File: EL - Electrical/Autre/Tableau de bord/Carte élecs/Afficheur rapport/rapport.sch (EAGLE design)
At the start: 15 parts, among them IC1 MCP23008P, X1 22-23-2041

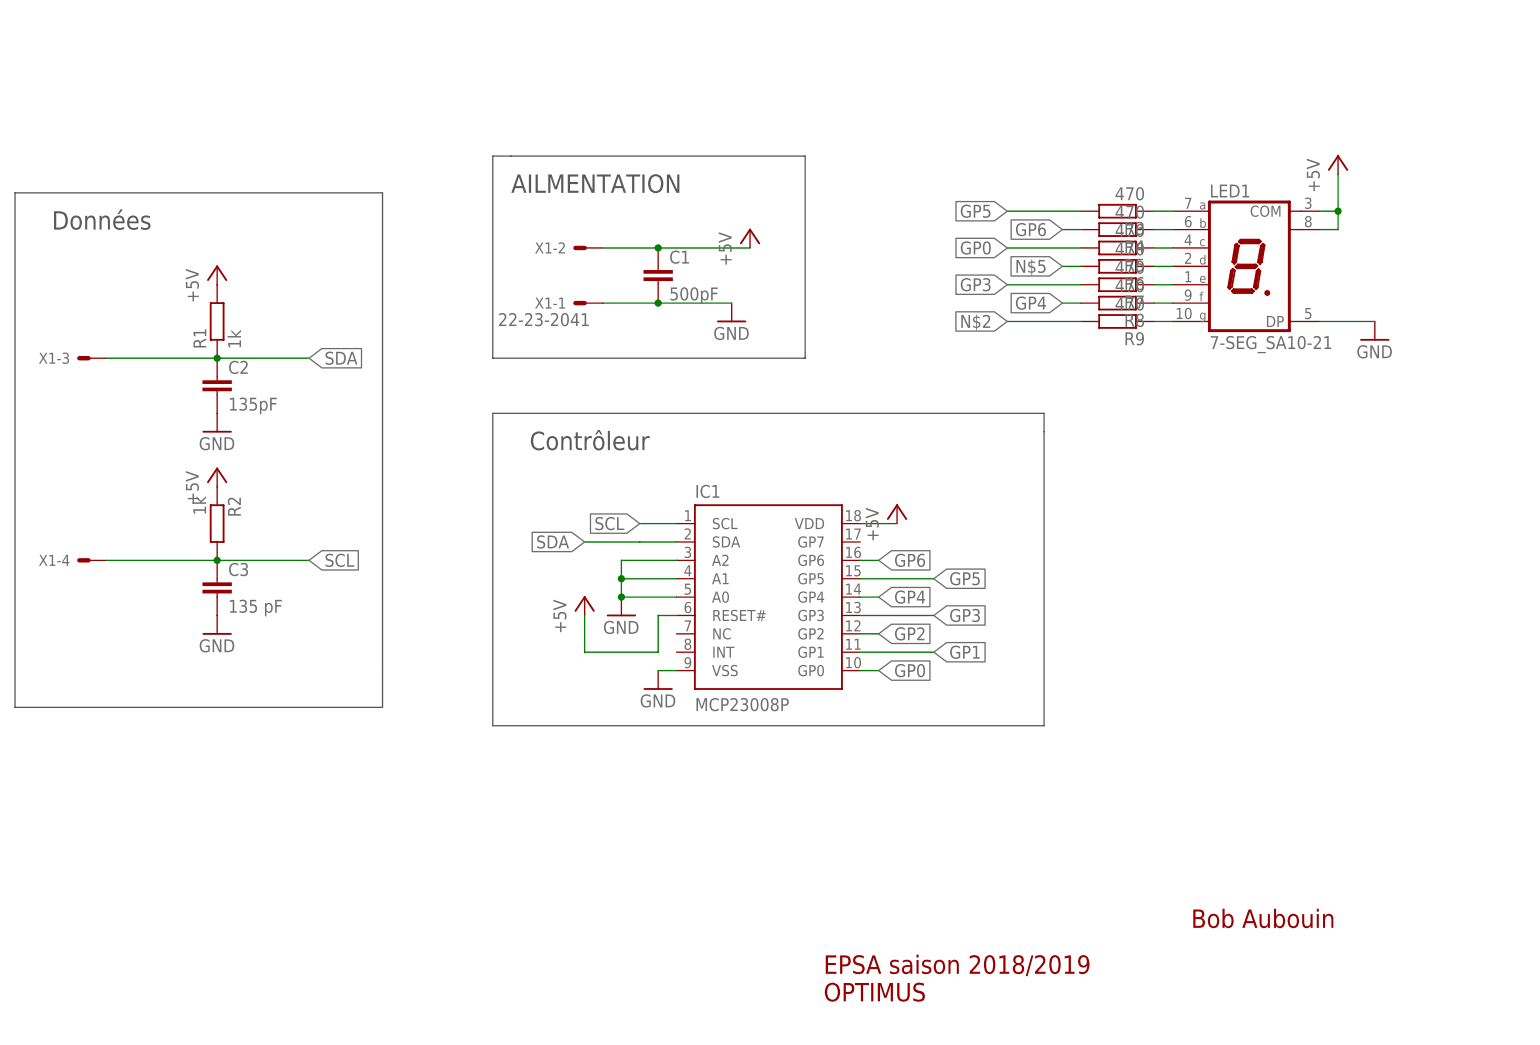
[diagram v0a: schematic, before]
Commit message: carte afficheur rapport et commandes
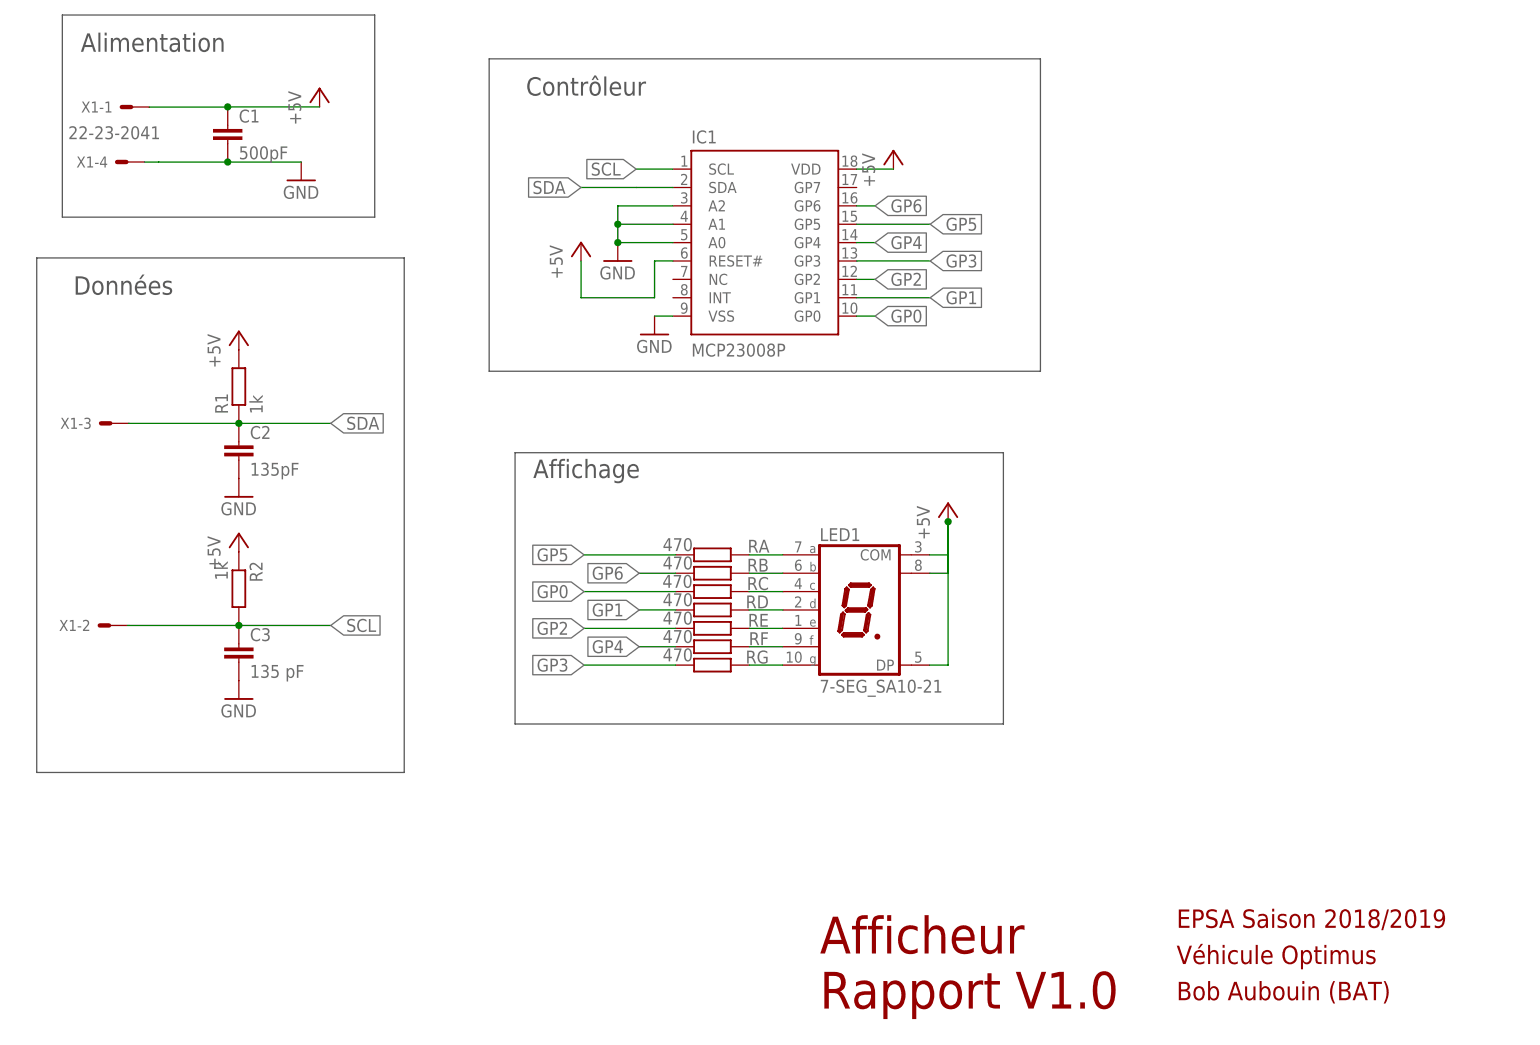
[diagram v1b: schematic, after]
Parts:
- removed R3, R4, R5, R6, R7, R8, R9: 470, rcl:R-EU_0204/7
- added RA, RB, RC, RD, RE, RF, RG: 470, rcl:R-EU_0204/7
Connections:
- removed net N$2: R9.2
- removed net N$5: R6.2
- net +5V: now also LED1.DP, X1-1.S; no longer X1-2.S
- net GND: now also X1-4.S; no longer LED1.DP, X1-1.S
- net GP0: now also RC.2; no longer R5.2
- net GP1: now also RD.2
- net GP2: now also RE.2
- net GP3: now also RG.2; no longer R7.2
- net GP4: now also RF.2; no longer R8.2
- net GP5: now also RA.2; no longer R3.2
- net GP6: now also RB.2; no longer R4.2
- net N$10: now also RG.1; no longer R9.1
- net N$11: now also RF.1; no longer R8.1
- net N$12: now also RE.1; no longer R7.1
- net N$13: now also RD.1; no longer R6.1
- net N$14: now also RC.1; no longer R5.1
- net N$15: now also RB.1; no longer R4.1
- net N$16: now also RA.1; no longer R3.1
- net SCL: now also X1-2.S; no longer X1-4.S
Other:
- note added: "Affichage"
- note added: "Afficheur Rapport V1.0"
- note added: "Alimentation"
- note added: "Bob Aubouin (BAT)"
- note added: "EPSA Saison 2018/2019"
- note added: "Véhicule Optimus"
- note removed: "AILMENTATION"
- note removed: "Bob Aubouin"
- note removed: "EPSA saison 2018/2019 OPTIMUS"
- moved on the sheet: C1, C2, C3, IC1, LED1, R1, R2, X1-1, X1-2, X1-3, X1-4
